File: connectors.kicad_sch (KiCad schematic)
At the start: 9 parts, among them J1 USB_C_Receptacle_USB2.0, J2 Motor_1_input, J3 Motor_2_input, J4 Power_Input, J5 Screw_Terminal_01x02, U3 USBLC6-2SC6

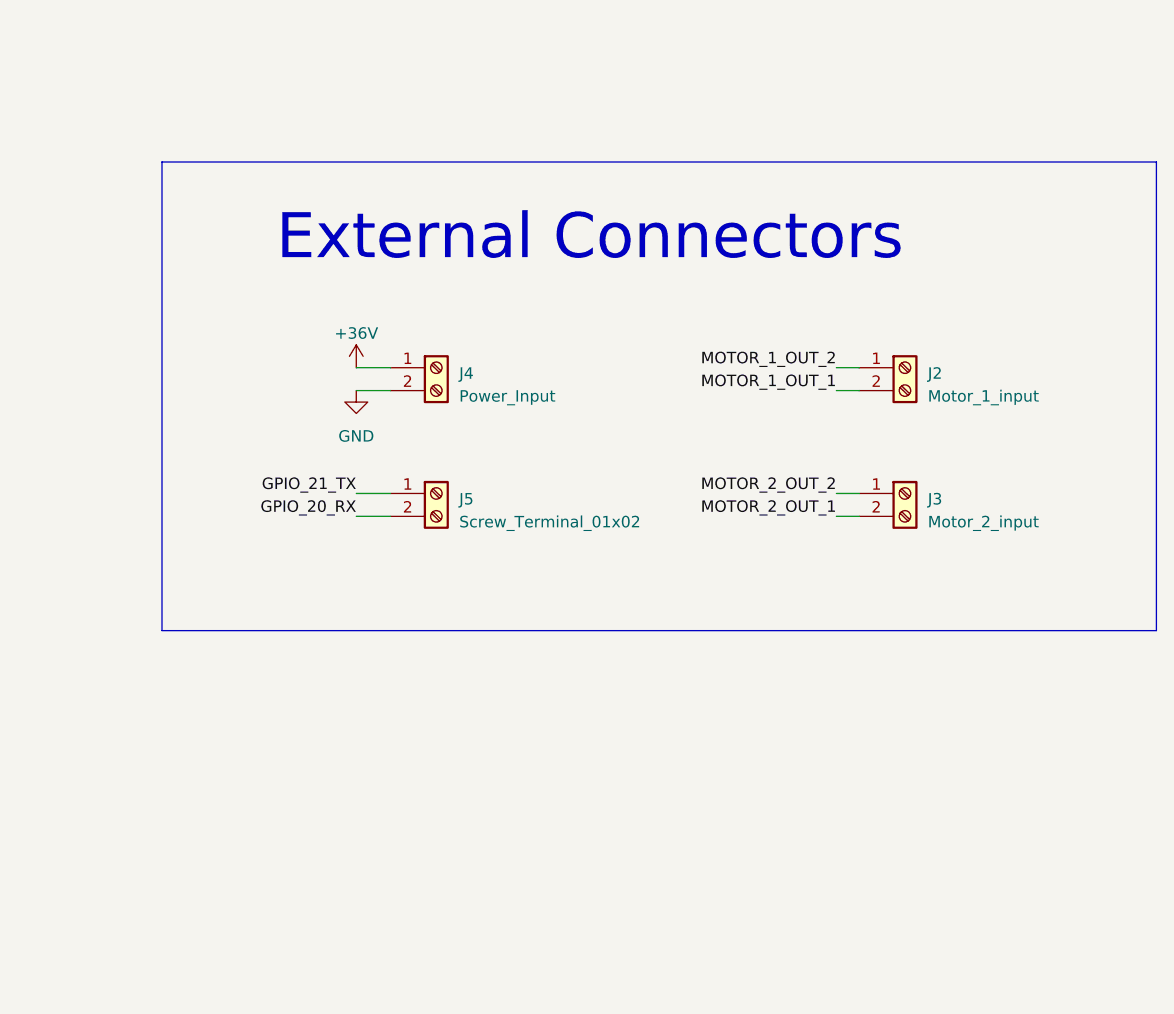
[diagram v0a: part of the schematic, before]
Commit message: Update placement
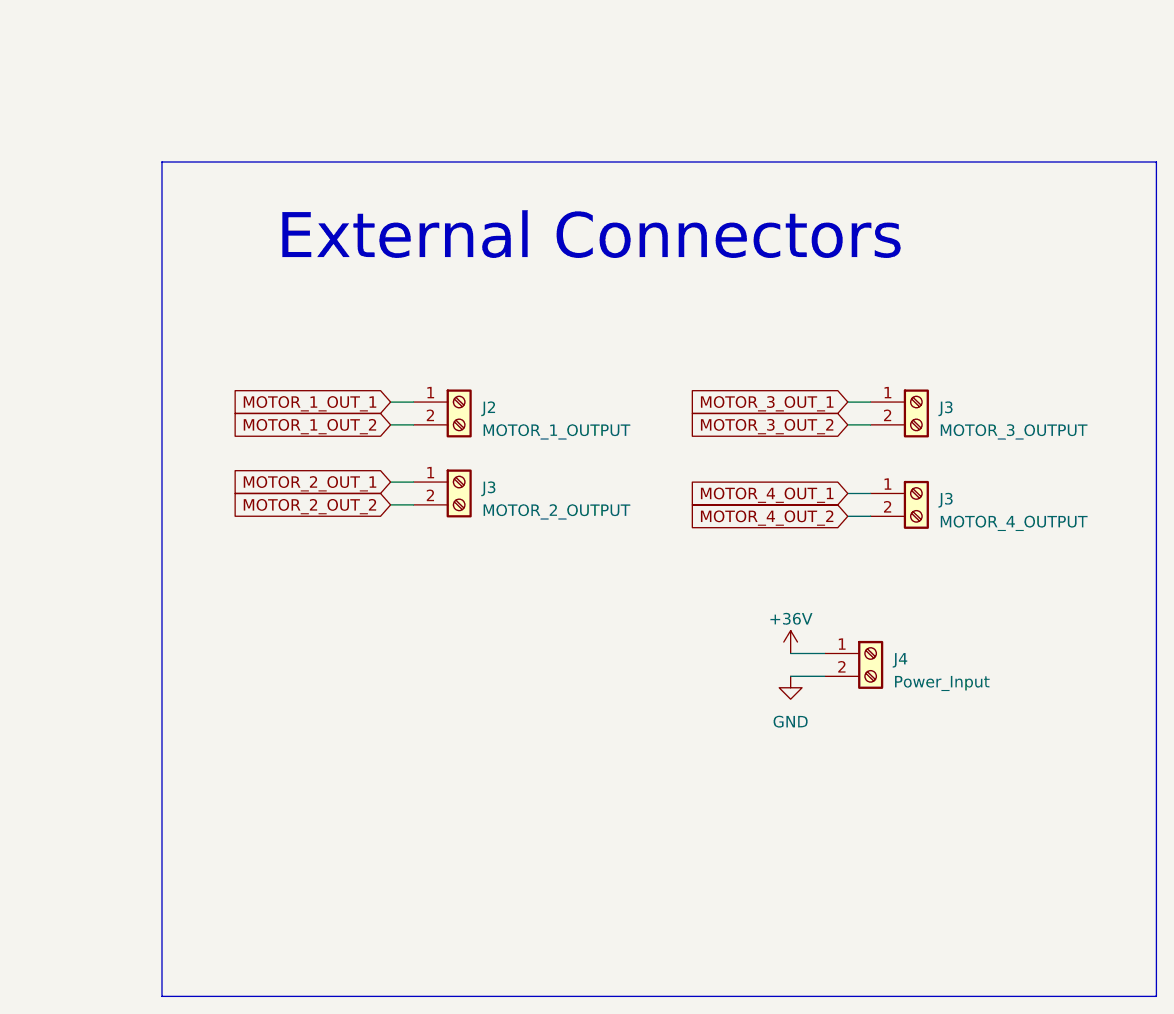
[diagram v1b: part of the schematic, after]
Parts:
- removed J5: Screw_Terminal_01x02, TerminalBlock:TerminalBlock_bornier-2_P5.08mm, symbol Connector:Screw_Terminal_01x02
- added J3: MOTOR_4_OUTPUT, TerminalBlock:TerminalBlock_bornier-2_P5.08mm, symbol Connector:Screw_Terminal_01x02
- added J3: MOTOR_3_OUTPUT, TerminalBlock:TerminalBlock_bornier-2_P5.08mm, symbol Connector:Screw_Terminal_01x02
- J2: value Motor_1_input -> MOTOR_1_OUTPUT
- J3: value Motor_2_input -> MOTOR_2_OUTPUT
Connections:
- net MOTOR_1_OUT_1: now also J2.1 (Pin_1); no longer J2.2 (Pin_2)
- net MOTOR_1_OUT_2: now also J2.2 (Pin_2); no longer J2.1 (Pin_1)
- net MOTOR_2_OUT_1: now also J3.1 (Pin_1); no longer J3.2 (Pin_2)
- net MOTOR_2_OUT_2: now also J3.2 (Pin_2); no longer J3.1 (Pin_1)
- new net MOTOR_3_OUT_1: J3.1 (Pin_1)
- new net MOTOR_3_OUT_2: J3.2 (Pin_2)
- new net MOTOR_4_OUT_1: J3.1 (Pin_1)
- new net MOTOR_4_OUT_2: J3.2 (Pin_2)
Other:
- moved on the sheet: J2, J3, J4
